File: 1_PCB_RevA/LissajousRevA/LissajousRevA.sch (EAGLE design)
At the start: 20 parts, among them U1 LM348D

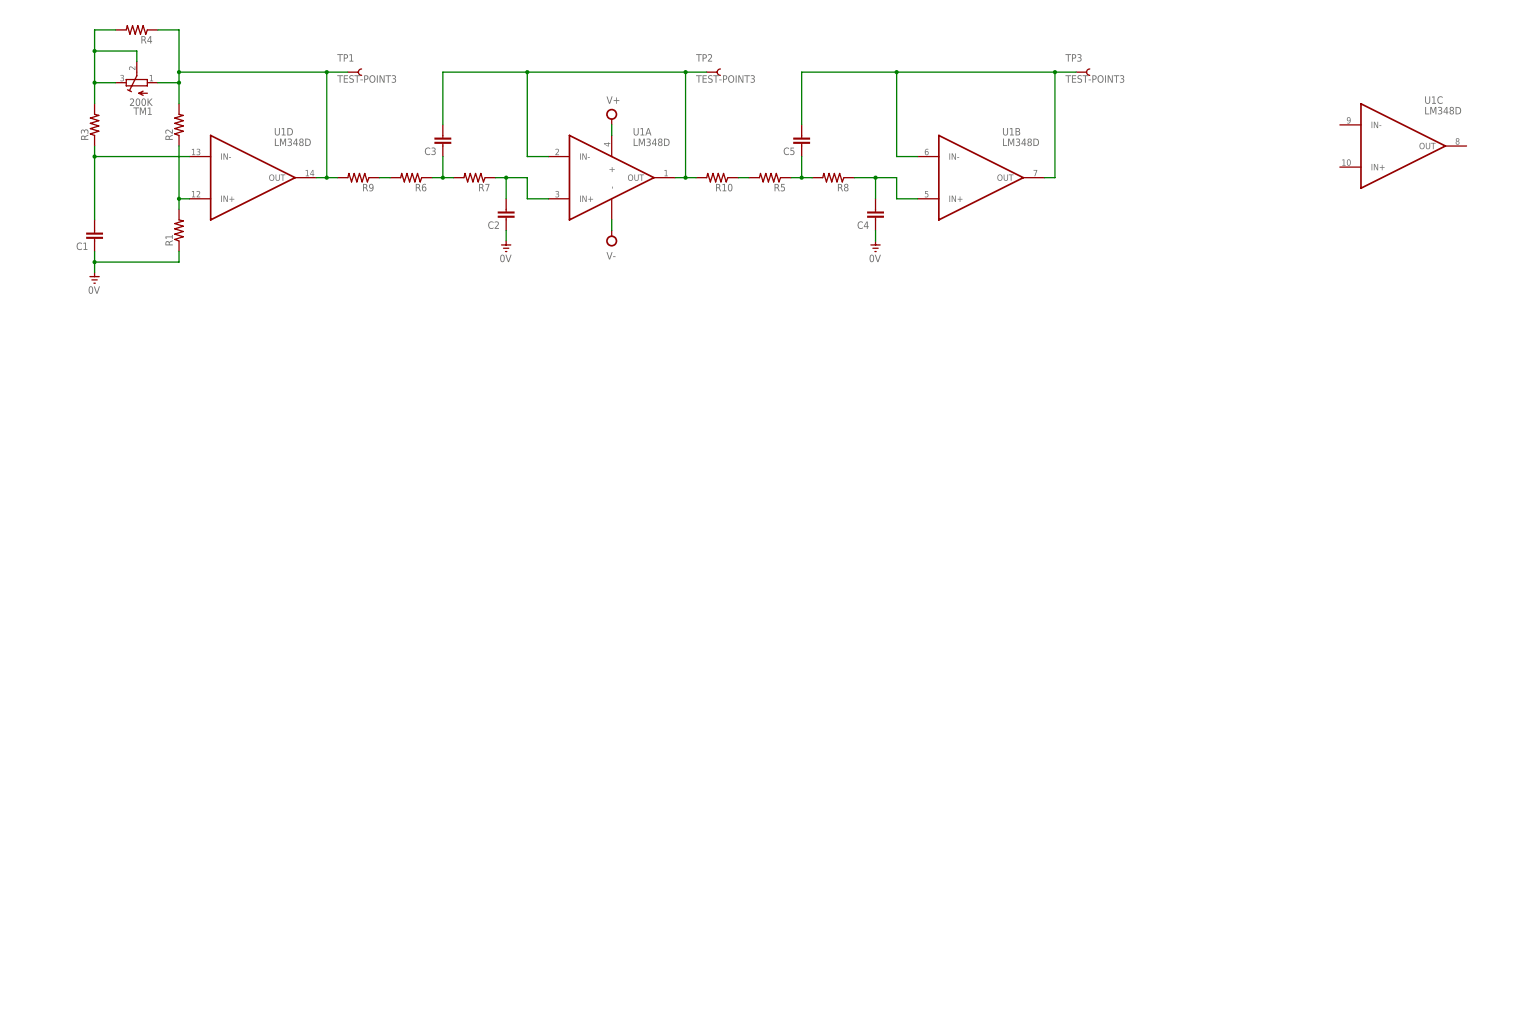
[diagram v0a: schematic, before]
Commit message: added second gen
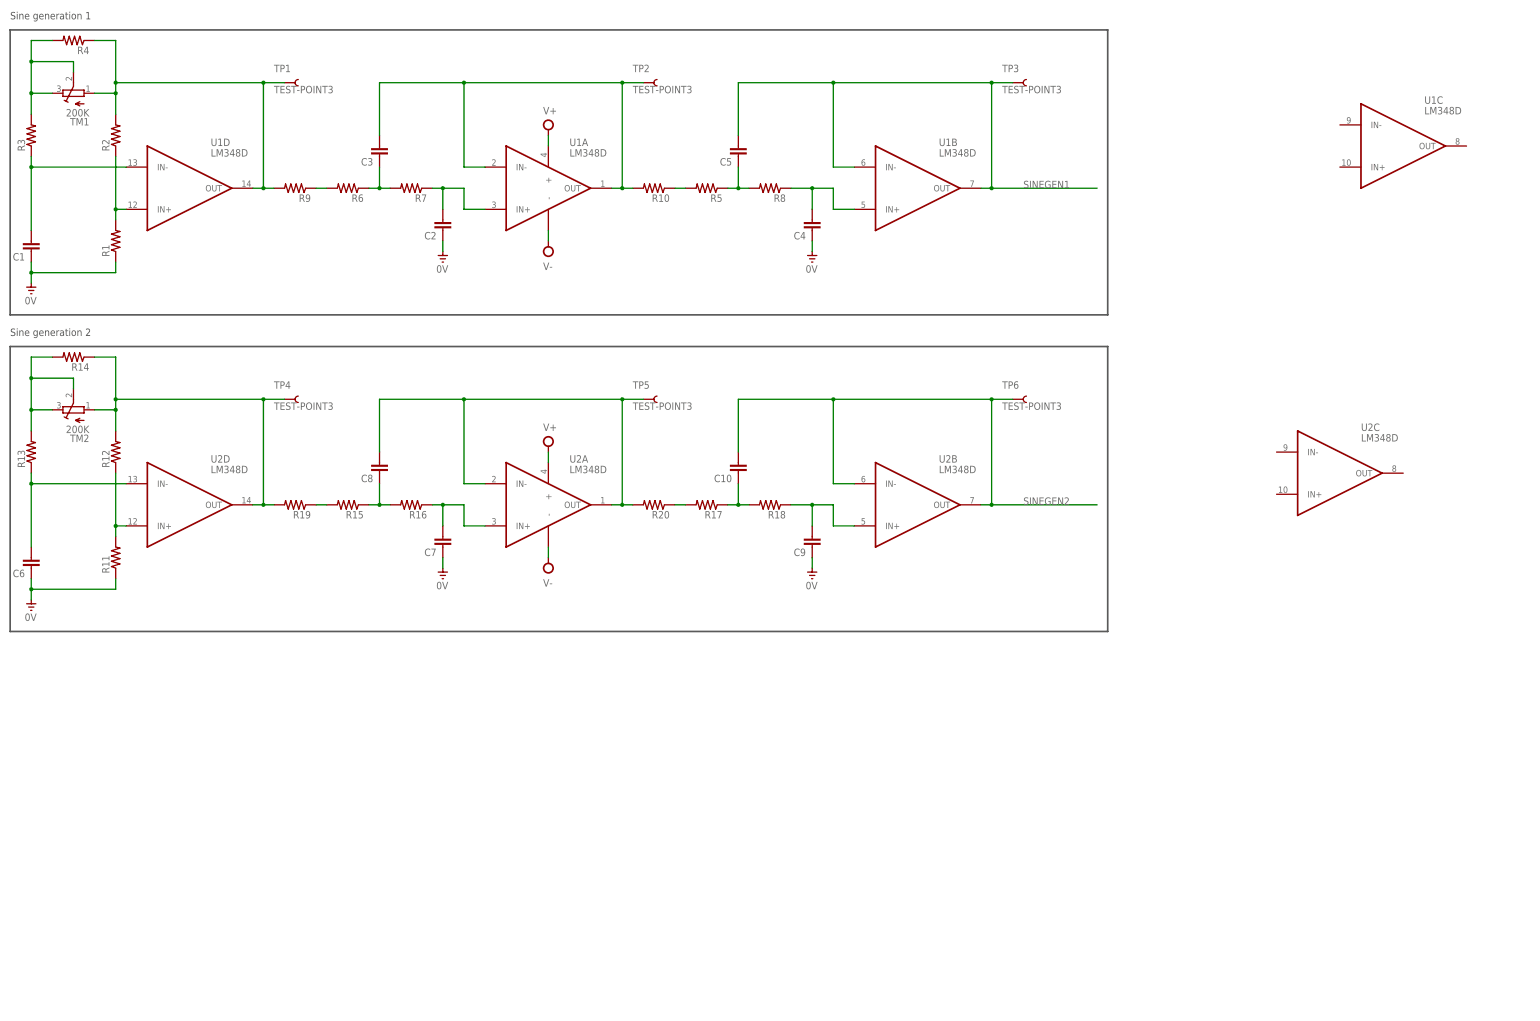
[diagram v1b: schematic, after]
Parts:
- added C10, C6, C7, C8, C9: (no value), passives:CAP0603-CAP
- added R11, R12, R13, R14, R15, R16, R17, R18, R19, R20: (no value), passives:RESISTOR0603-RES
- added TM2: 200K, adafruit:TRIMPOTTC33X
- added TP4, TP5, TP6: TEST-POINT3, passives:TEST-POINT3
- added U2: LM348D, LM348D:LM348D
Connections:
- net N$13 renamed SINEGEN1
- new net N$10: C6.2, R13.1, U2D.IN-
- new net N$15: R12.2, R14.1, R19.2, TM2.A, TP4.1, U2D.OUT
- new net N$16: C7.2, R16.1, U2A.IN+
- new net N$17: C8.1, R15.1, R16.2
- new net N$18: C9.2, R18.1, U2B.IN+
- new net N$19: C10.1, R17.1, R18.2
- new net N$21: C8.2, R20.2, TP5.1, U2A.IN-, U2A.OUT
- new net N$22: R15.2, R19.1
- new net N$23: R17.2, R20.1
- new net N$24: R13.2, R14.2, TM2.E, TM2.S
- new net N$9: R11.2, R12.1, U2D.IN+
- new net SINEGEN2: C10.2, TP6.1, U2B.IN-, U2B.OUT
- net 0V: now also C6.1, C7.1, C9.1, R11.1
- net V+: now also U2A.+
- net V-: now also U2A.-
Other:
- note added: "Sine generation 1"
- note added: "Sine generation 2"
- moved on the sheet: C1, C2, C3, C4, C5, R1, R10, R2, R3, R4, R5, R6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

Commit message: schmatics have everything down
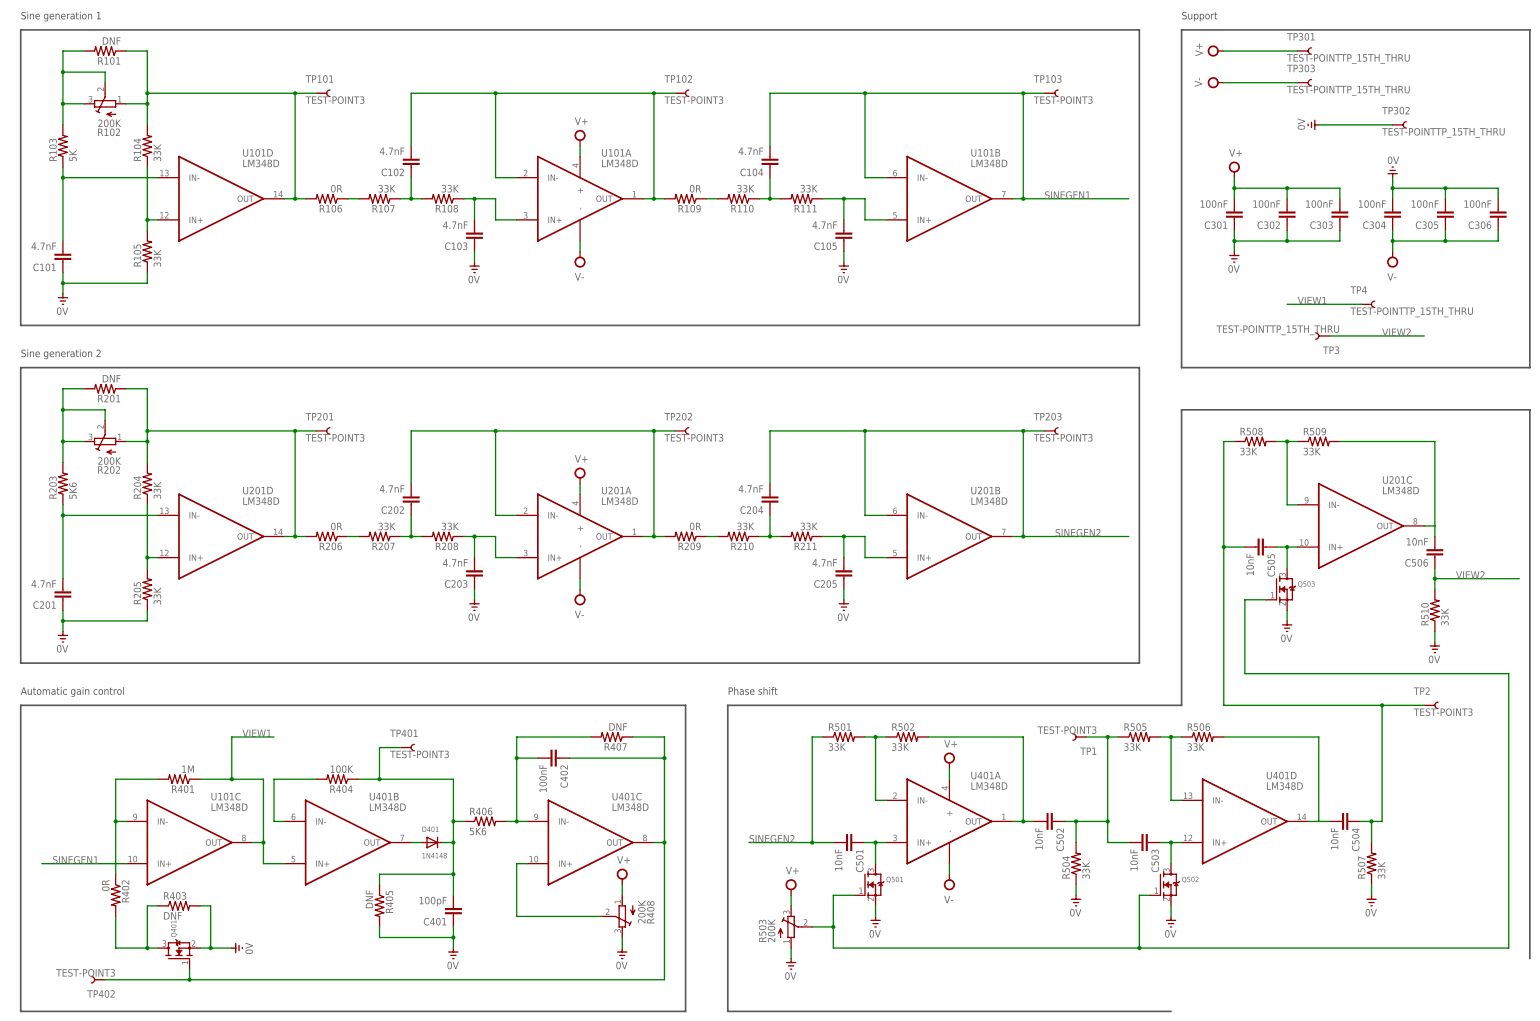
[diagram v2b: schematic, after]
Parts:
- removed C1, C10, C2, C3, C4, C5, C6, C7, C8, C9: (no value), passives:CAP0603-CAP
- removed R1, R10, R11, R12, R13, R14, R15, R16, R17, R18, R19, R2, R20, R3, R4, R5, R6, R7, R8, R9: (no value), passives:RESISTOR0603-RES
- removed TM1, TM2: 200K, adafruit:TRIMPOTTC33X
- removed TP5, TP6: TEST-POINT3, passives:TEST-POINT3
- removed U1, U2: LM348D, LM348D:LM348D
- added C101, C102, C103, C104, C105, C201, C202, C203, C204, C205: 4.7nF, passives:CAP0603-CAP
- added C301, C302, C303, C304, C305, C306, C402: 100nF, passives:CAP0603-CAP
- added C401: 100pF, passives:CAP0603-CAP
- added C501, C502, C503, C504, C505, C506: 10nF, passives:CAP0603-CAP
- added D401: 1N4148, adafruit:DIODESMA
- added Q401, Q501, Q502, Q503: (no value), adafruit:MOSFET-NREFLOW
- added R101, R201, R403, R405, R407: DNF, passives:RESISTOR0603-RES
- added R102, R202, R408, R503: 200K, adafruit:TRIMPOTTC33X
- added R103: 5K, passives:RESISTOR0603-RES
- added R104, R105, R107, R108, R110, R111, R204, R205, R207, R208, R210, R211, R501, R502, R504, R505, R506, R507, R508, R509, R510: 33K, passives:RESISTOR0603-RES
- added R106, R109, R206, R209, R402: 0R, passives:RESISTOR0603-RES
- added R203, R406: 5K6, passives:RESISTOR0603-RES
- added R401: 1M, passives:RESISTOR0603-RES
- added R404: 100K, passives:RESISTOR0603-RES
- added TP101, TP102, TP103, TP201, TP202, TP203, TP401, TP402: TEST-POINT3, passives:TEST-POINT3
- added TP301, TP302, TP303: TEST-POINTTP_15TH_THRU, passives:TEST-POINTTP_15TH_THRU
- added U101, U201, U401: LM348D, LM348D:LM348D
- TP3, TP4: value TEST-POINT3 -> TEST-POINTTP_15TH_THRU; device passives:TEST-POINT3 -> passives:TEST-POINTTP_15TH_THRU
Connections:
- new net N$13: R401.2, R402.1, U101C.IN-
- new net N$20: C501.1, Q501.D, U401A.IN+
- new net N$25: C402.2, R406.2, R407.2, U401C.IN-
- new net N$26: R501.2, R502.1, U401A.IN-
- new net N$27: R404.2, U401B.IN-
- new net N$28: D401.A, U401B.OUT
- new net N$29: C502.1, C503.2, R504.2, R505.1, TP1.1
- new net N$30: C401.2, D401.C, R404.1, R405.1, R406.1, TP401.1
- new net N$31: Q401.D, R402.2, R403.1
- new net N$32: C402.1, Q401.G, R407.1, TP402.1, U401C.OUT
- new net N$33: C502.2, R502.2, U401A.OUT
- new net N$34: R408.S, U401C.IN+
- new net N$35: C506.2
- new net N$36: C503.1, Q502.D, U401D.IN+
- new net N$37: R505.2, R506.1, U401D.IN-
- new net N$38: Q501.G, Q502.G, Q503.G, R503.S
- new net N$39: R506.2, U401D.OUT
- new net N$40: R508.2, R509.1, U201C.IN-
- new net N$41: C504.2
- new net N$42: C504.1, C505.2, R507.2, R508.1, TP2.1
- new net N$45: C505.1, Q503.D, U201C.IN+
- new net N$46: R509.2, U201C.OUT
- new net VIEW1: R401.1, TP4.1, U101C.OUT, U401B.IN+
- new net VIEW2: C506.1, R510.2, TP3.1
- net 0V: now also C101.1, C103.1, C105.1, C201.1, C203.1, C205.1, C301.1, C302.1, C303.1, C304.2, C305.2, C306.2, C401.1, Q401.S, Q501.S, Q502.S, Q503.S, R105.1, R205.1, R403.2, R405.2, R408.E, R503.A, R504.1, R507.1, R510.1, TP302.1; no longer C1.1, C2.1, C4.1, C6.1, C7.1, C9.1, R1.1, R11.1
- net N$1: now also C101.2, R103.1, U101D.IN-; no longer C1.2, R3.1, U1D.IN-
- net N$10: now also C201.2, R203.1, U201D.IN-; no longer C6.2, R13.1, U2D.IN-
- net N$11: now also C105.2, R111.1, U101B.IN+; no longer C4.2, R8.1, U1B.IN+
- net N$12: now also C104.1, R110.1, R111.2; no longer C5.1, R5.1, R8.2
- net N$14: now also R109.1, R110.2; no longer R10.1, R5.2
- net N$15: now also R201.1, R202.A, R204.2, R206.2, TP201.1, U201D.OUT; no longer R12.2, R14.1, R19.2, TM2.A, TP4.1, U2D.OUT
- net N$16: now also C203.2, R208.1, U201A.IN+; no longer C7.2, R16.1, U2A.IN+
- net N$17: now also C202.1, R207.1, R208.2; no longer C8.1, R15.1, R16.2
- net N$18: now also C205.2, R211.1, U201B.IN+; no longer C9.2, R18.1, U2B.IN+
- net N$19: now also C204.1, R210.1, R211.2; no longer C10.1, R17.1, R18.2
- net N$2: now also R104.1, R105.2, U101D.IN+; no longer R1.2, R2.1, U1D.IN+
- net N$21: now also C202.2, R209.2, TP202.1, U201A.IN-, U201A.OUT; no longer C8.2, R20.2, TP5.1, U2A.IN-, U2A.OUT
- net N$22: now also R206.1, R207.2; no longer R15.2, R19.1
- net N$23: now also R209.1, R210.2; no longer R17.2, R20.1
- net N$24: now also R201.2, R202.E, R202.S, R203.2; no longer R13.2, R14.2, TM2.E, TM2.S
- net N$3: now also R106.1, R107.2; no longer R6.2, R9.1
- net N$4: now also R101.2, R102.E, R102.S, R103.2; no longer R3.2, R4.2, TM1.E, TM1.S
- net N$5: now also C103.2, R108.1, U101A.IN+; no longer C2.2, R7.1, U1A.IN+
- net N$6: now also C102.1, R107.1, R108.2; no longer C3.1, R6.1, R7.2
- net N$7: now also R101.1, R102.A, R104.2, R106.2, TP101.1, U101D.OUT; no longer R2.2, R4.1, R9.2, TM1.A, TP1.1, U1D.OUT
- net N$8: now also C102.2, R109.2, TP102.1, U101A.IN-, U101A.OUT; no longer C3.2, R10.2, TP2.1, U1A.IN-, U1A.OUT
- net N$9: now also R204.1, R205.2, U201D.IN+; no longer R11.2, R12.1, U2D.IN+
- net SINEGEN1: now also C104.2, TP103.1, U101B.IN-, U101B.OUT, U101C.IN+; no longer C5.2, TP3.1, U1B.IN-, U1B.OUT
- net SINEGEN2: now also C204.2, C501.2, R501.1, TP203.1, U201B.IN-, U201B.OUT; no longer C10.2, TP6.1, U2B.IN-, U2B.OUT
- net V+: now also C301.2, C302.2, C303.2, R408.A, R503.E, TP301.1, U101A.+, U201A.+, U401A.+; no longer U1A.+, U2A.+
- net V-: now also C304.1, C305.1, C306.1, TP303.1, U101A.-, U201A.-, U401A.-; no longer U1A.-, U2A.-
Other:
- note added: "Automatic gain control"
- note added: "Phase shift"
- note added: "Support"
- moved on the sheet: TP1, TP2, TP3, TP4
